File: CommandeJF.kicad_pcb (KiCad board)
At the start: 2 copper layers, 100 x 70 mm, 15 parts, among them J1 Conn_01x04, J2 Conn_01x02, J3 Conn_01x04, K1 RelaisSRD, T1 Trou, T2 Trou, T3 Trou, T4 Trou, U1 DS3231, U101 MP1584

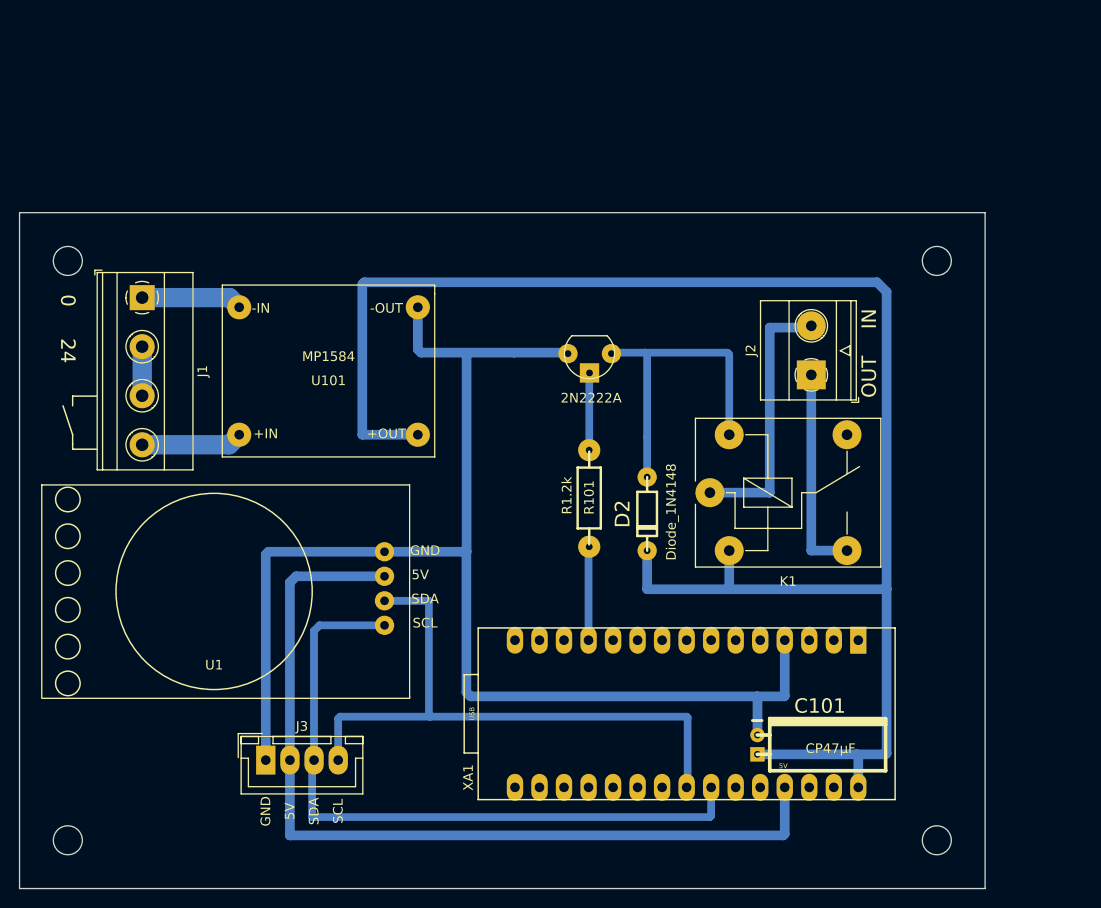
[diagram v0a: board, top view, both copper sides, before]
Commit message: version 1
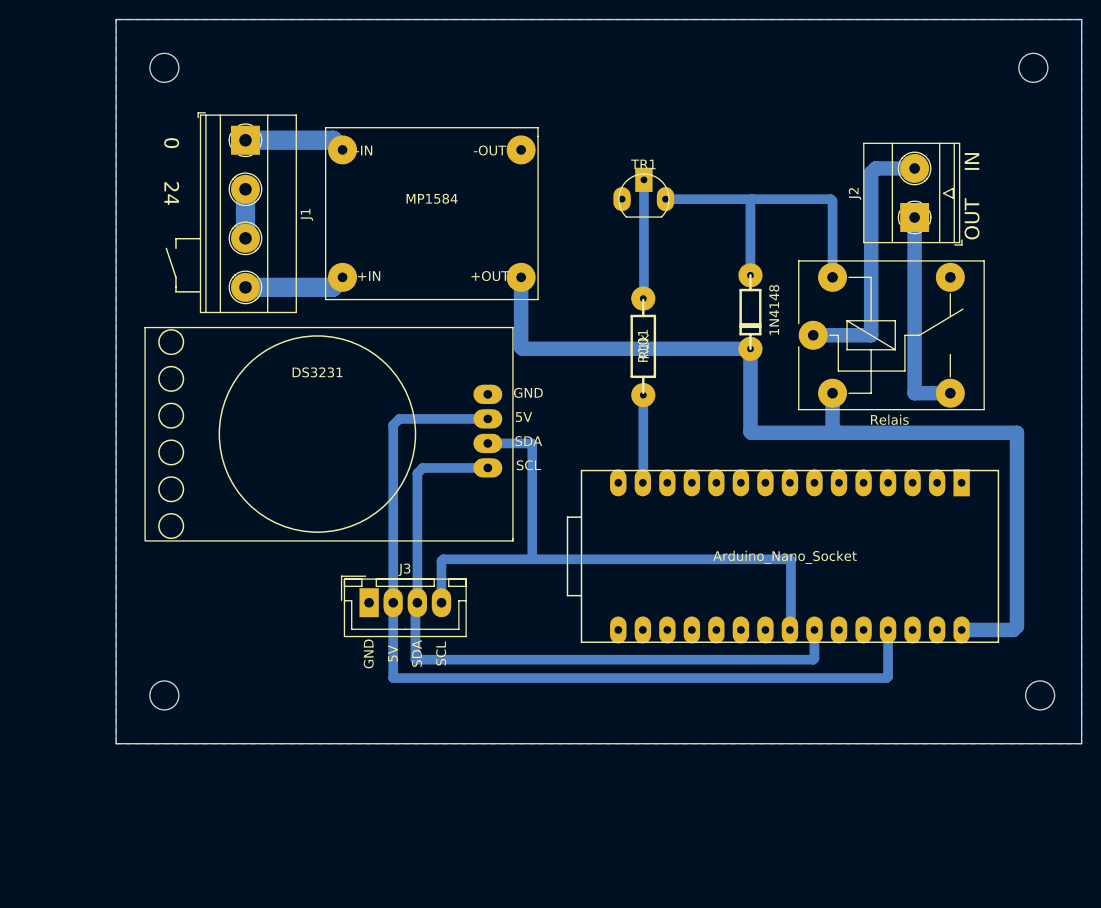
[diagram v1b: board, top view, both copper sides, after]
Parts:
- removed C101: CP47µF, capacitors:CP_5x11mm_hor
- D2: value Diode_1N4148 -> 1N4148
- K1: value RelaisSRD -> Relais
- R101: value R1.2k -> R1k
- TR1: value 2N2222A -> Transistor_TO92
- moved D2 23.5 mm to (170.7, 65.3)
- moved T1 22.4 mm to (110.0, 40.0)
- moved T2 22.4 mm to (200.0, 40.0)
- moved XA1 19.5 mm to (153.2, 90.6)
- moved J1 19.5 mm to (118.4, 47.5)
- moved U1 19.5 mm to (125.8, 77.9)
- moved U101 19.5 mm to (137.7, 55.1)
- moved J2 19.5 mm to (187.7, 55.5)
- moved J3 19.5 mm to (131.2, 95.4)
- moved K1 19.5 mm to (177.2, 67.7)
- moved T4 18.4 mm to (200.7, 105.0)
- moved T3 18.0 mm to (110.0, 105.0)
- moved R101 16.7 mm to (159.7, 69.0)
- moved TR1 16.3 mm to (158.4, 53.6), turned to 0 degrees
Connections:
- TR1 pad 1: Net-(D2-Pad2) -> GND
- TR1 pad 3: GND -> Net-(D2-Pad2)
- XA1 pad D11: (no net) -> SIG
- XA1 pad D9: SIG -> (no net)
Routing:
- net GND: track 140.4 -> 0.00 mm
- net +12V: track 173.7 -> 97.7 mm
- net Net-(R101-Pad1): track 8.01 -> 12.3 mm
- net SIG: track 9.71 -> 9.10 mm
- added copper zone on B.Cu, net GND
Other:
- board size 100 x 70 mm -> 100 x 75 mm
- net class 12V: trace_width 1 -> 1.5
- net class Default: trace_width 0.8 -> 1
